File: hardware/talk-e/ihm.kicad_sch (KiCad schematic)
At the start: 32 parts, among them J1 Conn_01x04_Socket, J2 Conn_01x02_Socket, J3 Conn_02x04_Odd_Even, J4 Conn_Coaxial, Q2 BC337, SW1 SW_Push, SW2 SW_Push, SW3 SW_Push, SW5 SW_Push, U1 RFM96W-433S2, U4 ESP32-S3, Y1 Crystal

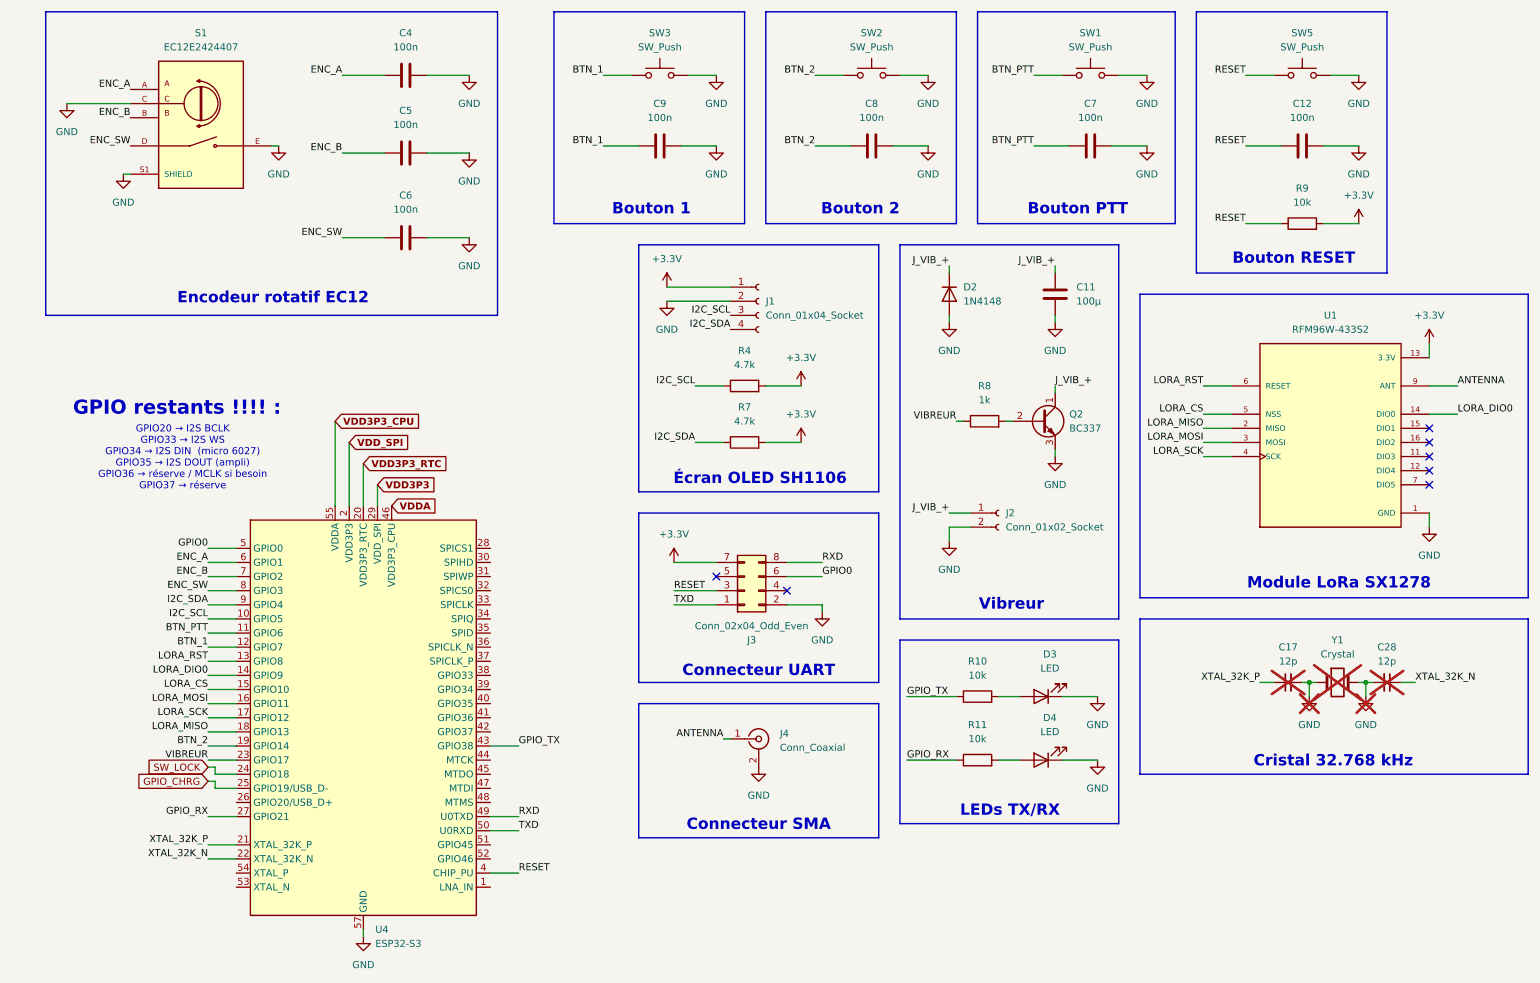
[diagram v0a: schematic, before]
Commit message: Something moved in the schematic but idk what
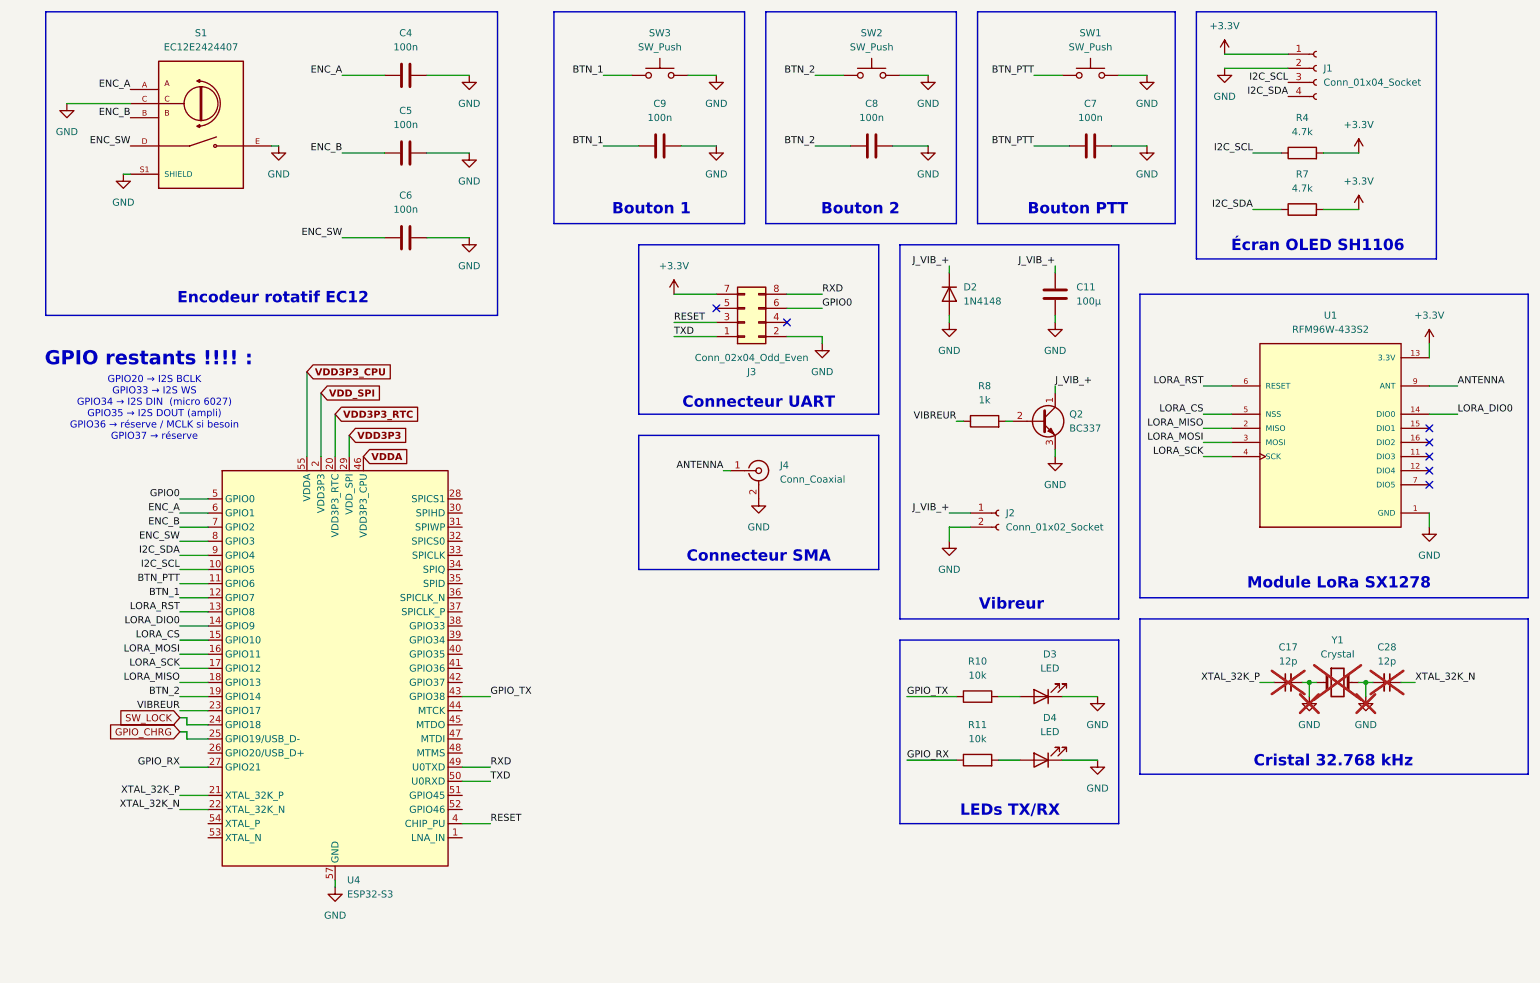
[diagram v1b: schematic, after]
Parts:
- removed C12: 100n, symbol Device:C
- removed R9: 10k, symbol Device:R
- removed SW5: SW_Push, symbol Switch:SW_Push
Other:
- note removed: "Bouton RESET"
- moved on the sheet: J1, J3, J4, R4, R7, U4
